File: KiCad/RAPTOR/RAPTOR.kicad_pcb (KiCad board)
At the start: 2 copper layers, 138.4 x 101.6 mm, 28 parts, among them J1 SOLC_CONN, J10 EXT_LED3, J11 SRVOL_CONN, J12 SRVOR_CONN, J14 RBF_CONN, J15 EEP_BTN_CONN, J18 CONN_BUZZER, J2 SOLP_CONN, J3 POWER, J4 CONN_LED_FIX, J7 EXT_LED0, J8 EXT_LED1, J9 EXT_LED2, Q1 SOLC_MSFT, Q2 SOLC_MSFT, Q3 BZZ_MSFT, Q4 LED_MSFT, U1 BMP280 Breakout, U2 BNO055 Breakout, U3 OpenLog, U4 AdafruitGPS, U5 Teensy3.2, U6 D24V550F5

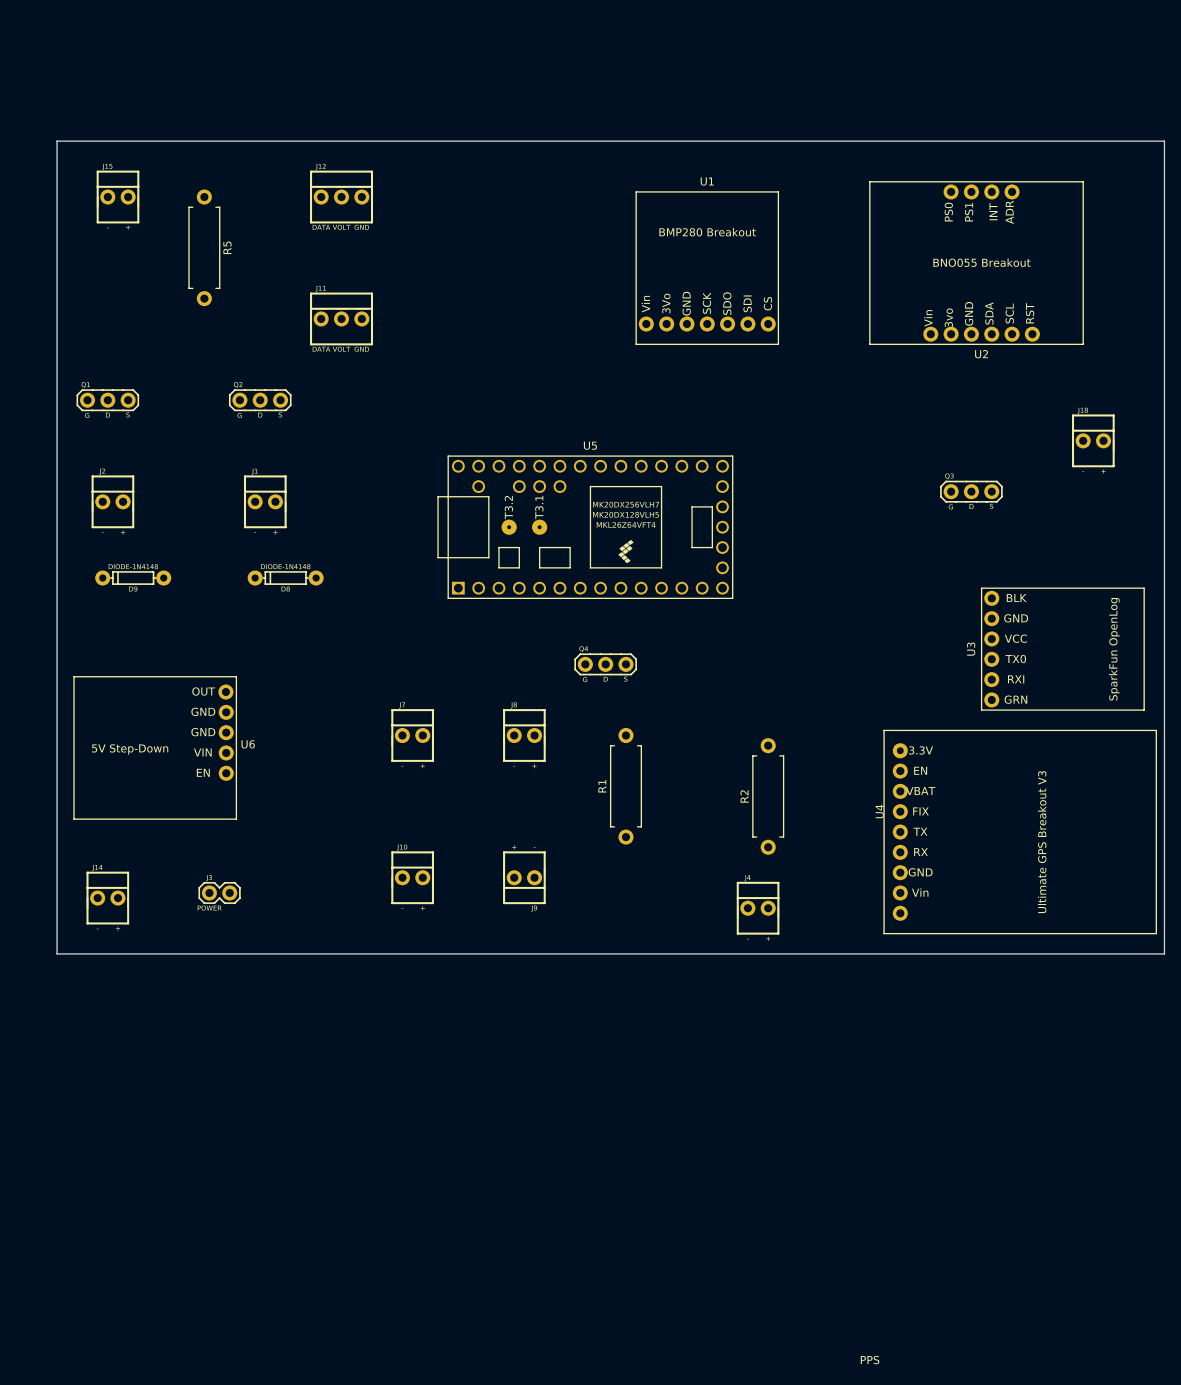
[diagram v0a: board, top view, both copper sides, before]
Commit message: Routed The Headder
Got the pins where I wanted them to make routing easeir
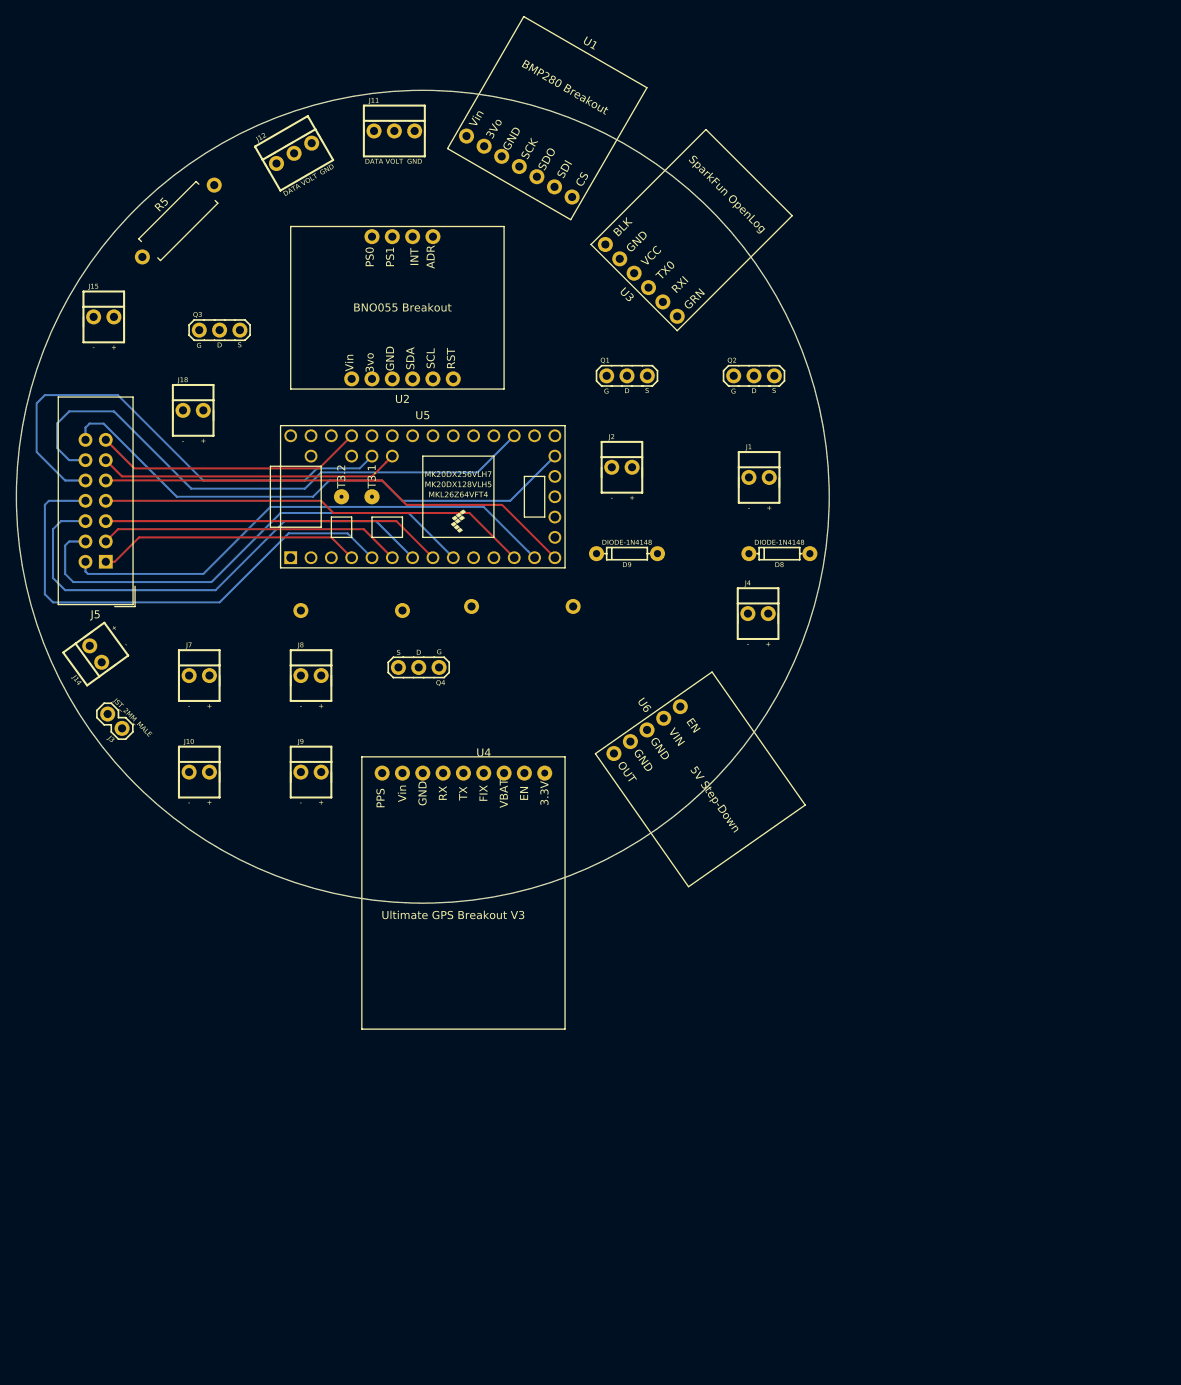
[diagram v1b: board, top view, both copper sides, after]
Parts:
- added J5: EXTENSION_HEADER, Connector_IDC:IDC-Header_2x07_P2.54mm_Vertical, F.Cu at (100.1, 97.0)
- J3: value POWER -> JST_2MM_MALE
- Q1, Q2: value SOLC_MSFT -> MOSFET-NCH-STQ2NK60ZR-AP
- Q3: value BZZ_MSFT -> MOSFET-NCH-STQ2NK60ZR-AP
- Q4: value LED_MSFT -> MOSFET-NCH-STQ2NK60ZR-AP
- R1, R2: moved to B.Cu
- moved J18 112.6 mm to (109.7, 78.7)
- moved Q3 96.1 mm to (111.8, 68.1)
- moved U2 72.6 mm to (137.2, 74.2)
- moved Q1 65.0 mm to (162.7, 73.8)
- moved U3 63.9 mm to (166.1, 61.0), turned to 315 degrees
- moved J2 63.8 mm to (163.3, 85.9)
- moved U6 62.4 mm to (175.3, 113.8), turned to 215 degrees
- moved D9 61.8 mm to (165.2, 96.0)
- moved J1 61.8 mm to (180.5, 87.1)
- moved Q2 61.8 mm to (178.6, 73.8)
- moved D8 61.8 mm to (184.3, 96.0)
- moved U4 55.1 mm to (144.8, 123.4), turned to 180 degrees
- moved R1 49.5 mm to (124.5, 103.1), turned to 0 degrees
- moved R2 38.7 mm to (158.5, 102.6), turned to 180 degrees
- moved J4 36.8 mm to (180.3, 104.1)
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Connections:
- J11 pad 1: Net-(J11-Pad1) -> /SRVO_L
- J12 pad 1: Net-(J12-Pad1) -> /SRVO_R
- R5 pad 2: Net-(R5-Pad2) -> GND
- U5 pad 12: Net-(U5-Pad12) -> /PIN_10
- U5 pad 13: Net-(U5-Pad13) -> /PIN_11
- U5 pad 14: Net-(U5-Pad14) -> /PIN_12
- U5 pad 19: Net-(U5-Pad19) -> /PIN_A14
- U5 pad 22: /HOTWIRE -> /PIN_15
- U5 pad 30: Net-(U5-Pad30) -> /PIN_23
- U5 pad 31: Net-(U5-Pad31) -> +3V3
- U5 pad 36: Net-(U5-Pad36) -> /PIN_A10
- U5 pad 37: Net-(U5-Pad37) -> /PIN_A11
- U5 pad 4: Net-(U5-Pad4) -> /PIN_2
- U5 pad 5: Net-(U5-Pad5) -> /PIN_3
- U5 pad 6: Net-(U5-Pad6) -> /PIN_4
- U5 pad 7: Net-(U5-Pad7) -> /PIN_5
- U5 pad 8: Net-(U5-Pad8) -> /PIN_6
- U5 pad 9: Net-(U5-Pad9) -> /PIN_7
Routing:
- net /PIN_15: track 0.00 -> 71.7 mm
- net /PIN_A14: track 0.00 -> 68.4 mm
- net /PIN_11: track 0.00 -> 63.6 mm
- net /PIN_3: track 0.00 -> 62.6 mm
- net /PIN_A10: track 0.00 -> 61.7 mm
- net /PIN_5: track 0.00 -> 61.6 mm
- net /PIN_7: track 0.00 -> 61.1 mm
- net /PIN_12: track 0.00 -> 60.1 mm
- net /PIN_10: track 0.00 -> 54.0 mm
- net /PIN_6: track 0.00 -> 42.8 mm
- net /PIN_4: track 0.00 -> 37.9 mm
- net /PIN_A11: track 0.00 -> 37.7 mm
- net /PIN_23: track 0.00 -> 33.9 mm
- net /PIN_2: track 0.00 -> 33.0 mm
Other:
- board size 138.4 x 101.6 mm -> 101.6 x 101.6 mm
